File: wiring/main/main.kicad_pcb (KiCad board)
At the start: 2 copper layers, 90 x 50 mm, 16 parts

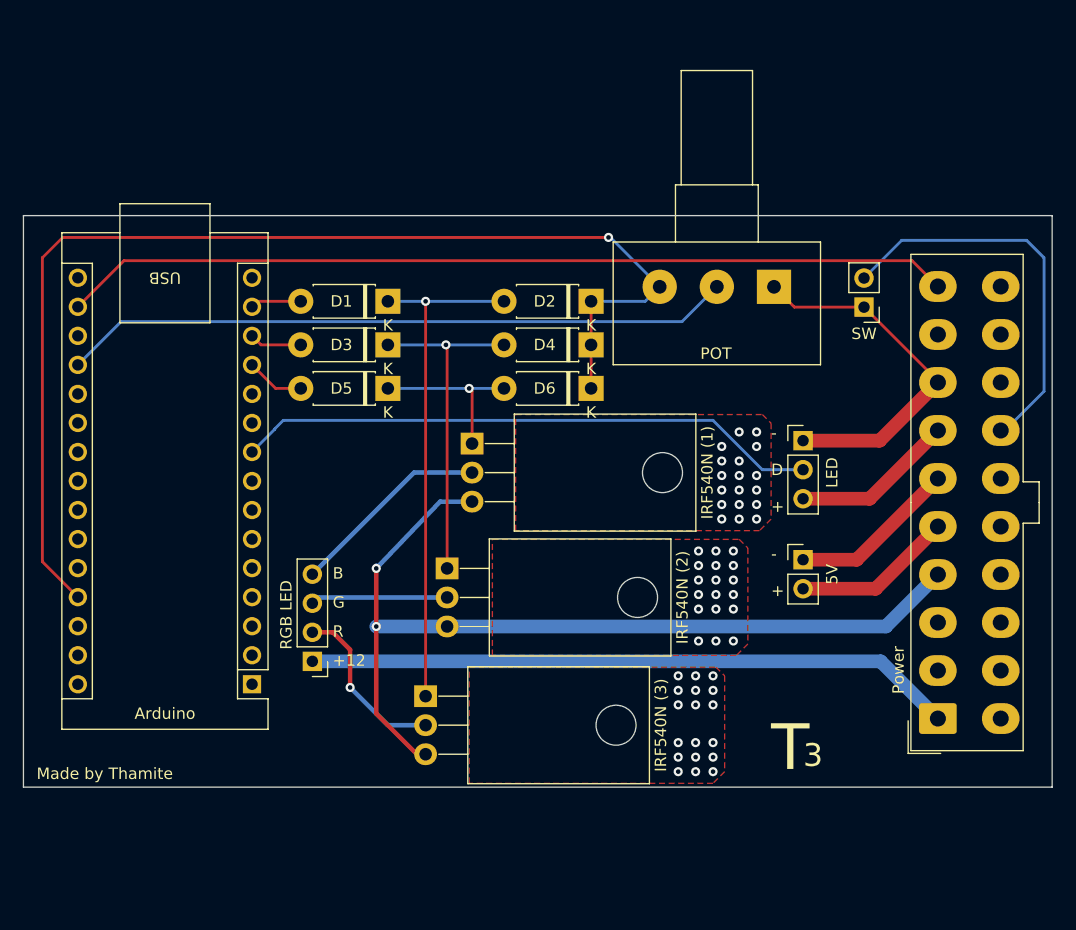
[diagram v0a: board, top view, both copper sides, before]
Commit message: basic implémentation of the last commit
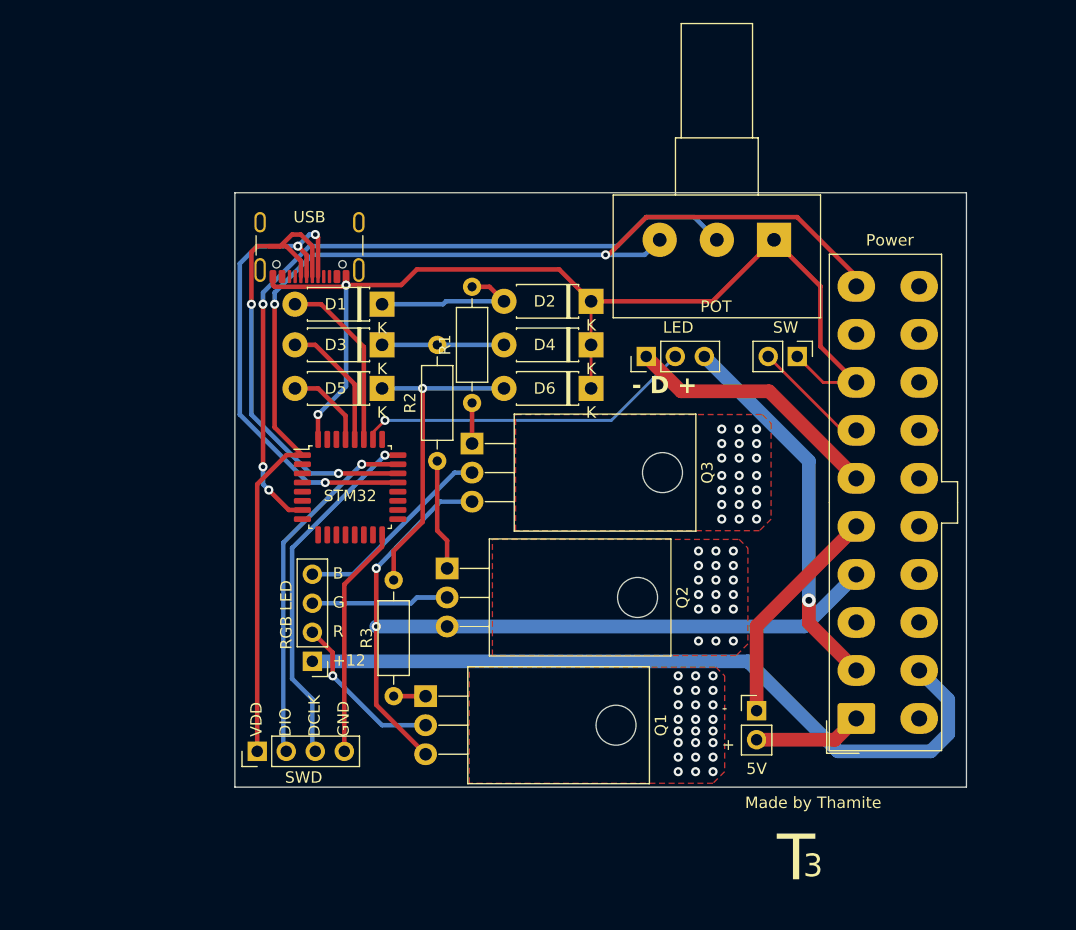
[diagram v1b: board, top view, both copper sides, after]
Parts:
- removed Arduino: Arduino_Nano, Module:Arduino_Nano
- added R1: R_Axial_DIN0207_L6.3mm_D2.5mm_P10.16mm_Horizontal, Resistor_THT:R_Axial_DIN0207_L6.3mm_D2.5mm_P10.16mm_Horizontal, F.Cu at (79.2, 56.4)
- added R2: R_Axial_DIN0207_L6.3mm_D2.5mm_P10.16mm_Horizontal, Resistor_THT:R_Axial_DIN0207_L6.3mm_D2.5mm_P10.16mm_Horizontal, F.Cu at (76.2, 61.5)
- added R3: R_Axial_DIN0207_L6.3mm_D2.5mm_P10.16mm_Horizontal, Resistor_THT:R_Axial_DIN0207_L6.3mm_D2.5mm_P10.16mm_Horizontal, F.Cu at (72.4, 82.0)
- added STM32: LQFP-32_7x7mm_P0.8mm, Package_QFP:LQFP-32_7x7mm_P0.8mm, F.Cu at (68.6, 63.8)
- added SWD: PinHeader_1x04_P2.54mm_Vertical, Connector_PinHeader_2.54mm:PinHeader_1x04_P2.54mm_Vertical, F.Cu at (60.5, 86.9)
- added USB: USB_C_Receptacle_GCT_USB4105-xx-A_16P_TopMnt_Horizontal, Connector_USB:USB_C_Receptacle_GCT_USB4105-xx-A_16P_TopMnt_Horizontal, F.Cu at (65.0, 41.7)
- Q1: renamed from IRF540N (3)
- Q2: renamed from IRF540N (2)
- Q3: renamed from IRF540N (1)
- moved LED 15.6 mm to (94.5, 52.3), turned to 90 degrees
- moved 5V 13.8 mm to (104.1, 83.3)
- moved SW 7.26 mm to (107.7, 52.3), turned to -90 degrees
- moved Power 7.14 mm to (112.9, 84.0)
- moved POT 4.11 mm to (105.7, 42.1)
- moved D1 0.57 mm to (71.4, 47.8)
- moved D3 0.51 mm to (71.4, 51.3)
- moved D5 0.51 mm to (71.4, 55.1)
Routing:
- net (no net): track 685.4 -> 844.1 mm, vias 7 -> 20
- net PAD3: vias 18 -> 24
- net PAD1: vias 18 -> 21
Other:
- board size 90 x 50 mm -> 64 x 52 mm
- board text added: "DCLK"
- board text added: "DIO"
- board text added: "GND"
- board text added: "VDD"
